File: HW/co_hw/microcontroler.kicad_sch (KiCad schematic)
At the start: 31 parts, among them J7 Programmer, SW1 RotaryEncoder_Switch, SW2 SW_DIP_x03, SW3 SW_Push, U1 STM32F103C8Tx, U6 W25Q32JVSS, Y1 8Mhz

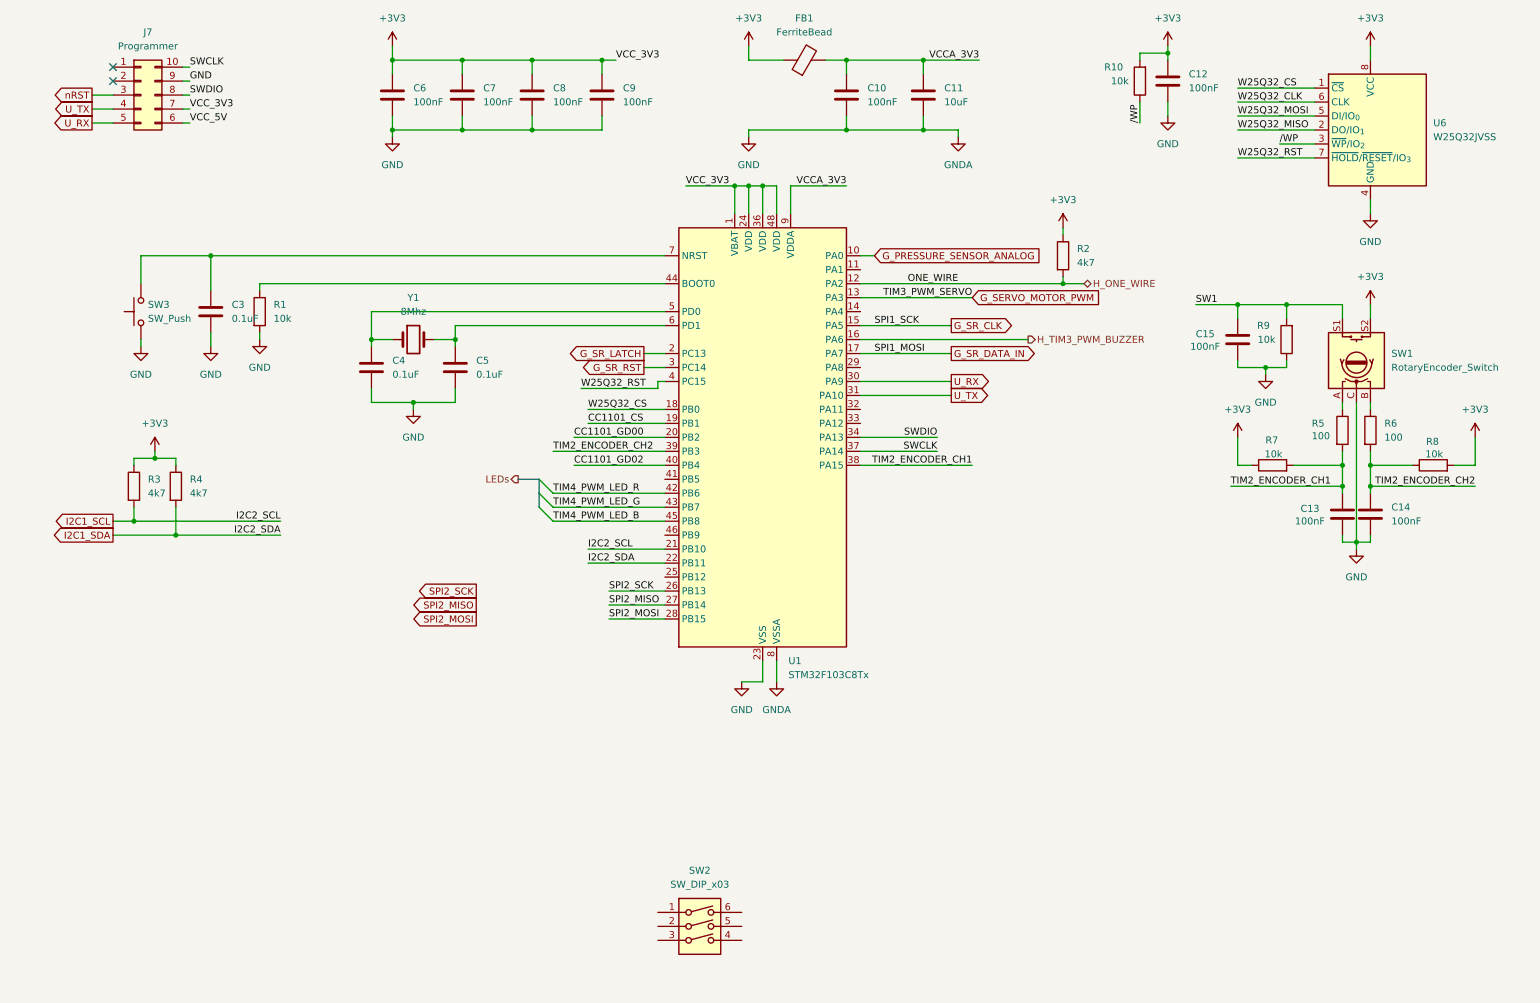
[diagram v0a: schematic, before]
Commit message: HW update
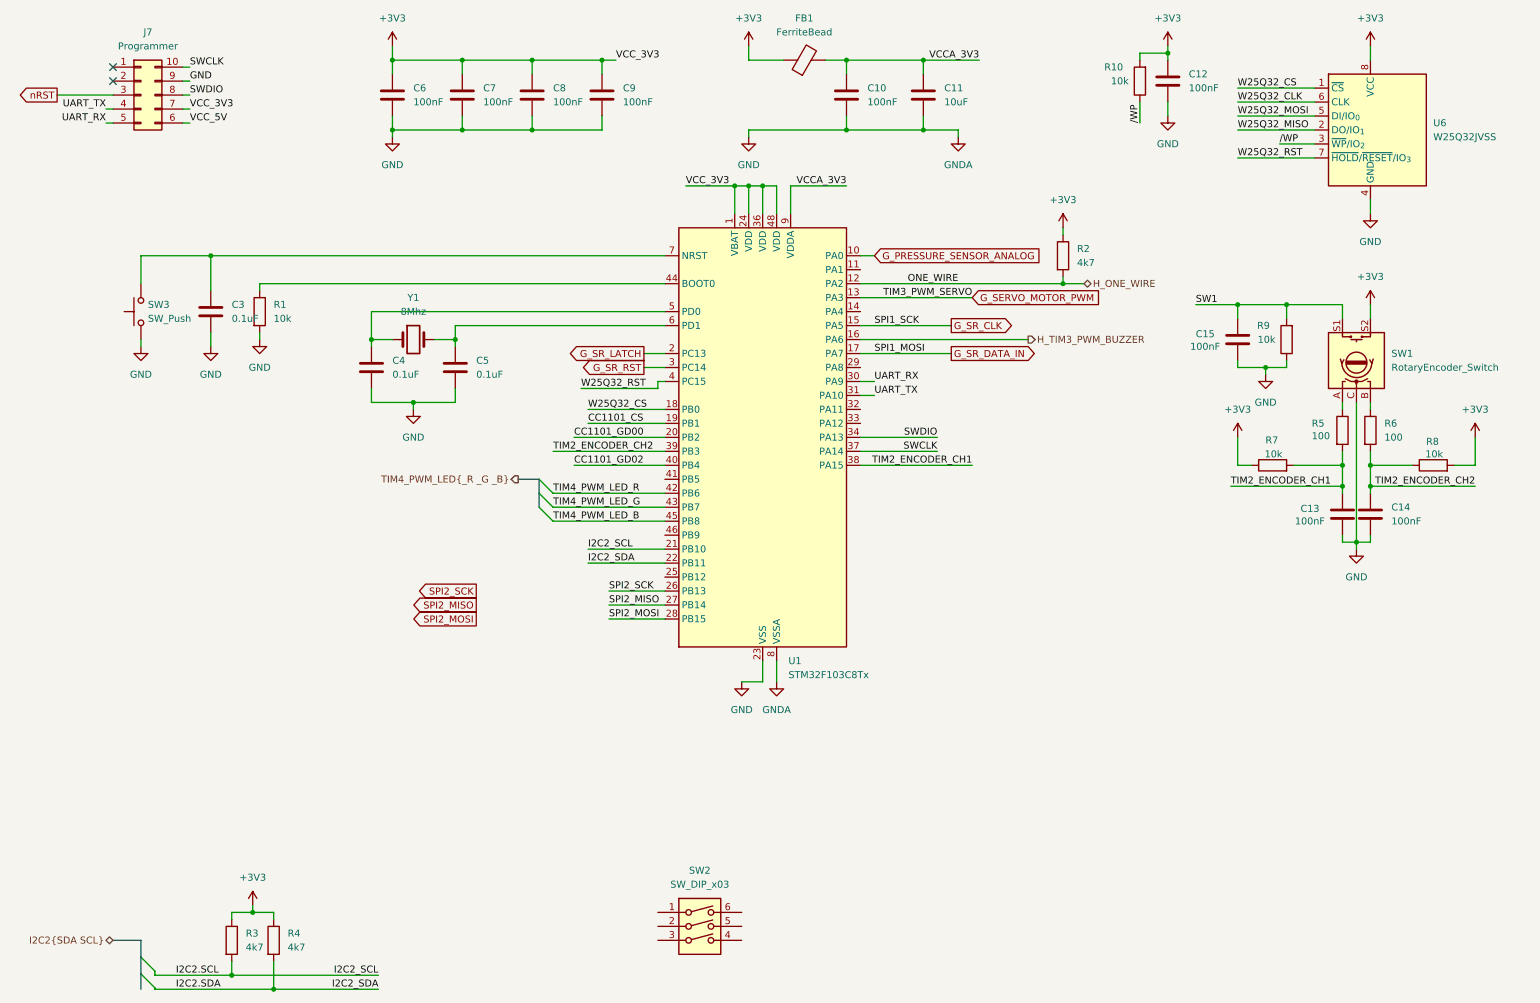
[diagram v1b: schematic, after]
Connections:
- net I2C1_SCL renamed I2C2.SCL
- net I2C1_SDA renamed I2C2.SDA
- net U_RX renamed UART_RX
- net U_TX renamed UART_TX
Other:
- moved on the sheet: R3, R4
